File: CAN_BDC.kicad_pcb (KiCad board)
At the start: 2 copper layers, 24.5 x 34 mm, 31 parts, among them P1 CONN_01X02, P2 CONN_01X05, P4 CONN_01X04, P5 CONN_01X04, P6 CONN_01X02, P7 CONN_01X04, P8 CONN_01X04, P9 CONN_01X02, U1 PSD2CAN, U2 SN65HVD232D, U3 POLOLU_DRV8825/DRV8801, U4 STM32F042G4U6, U5 Mini-360, U6 MCP1700T-3302E/TT

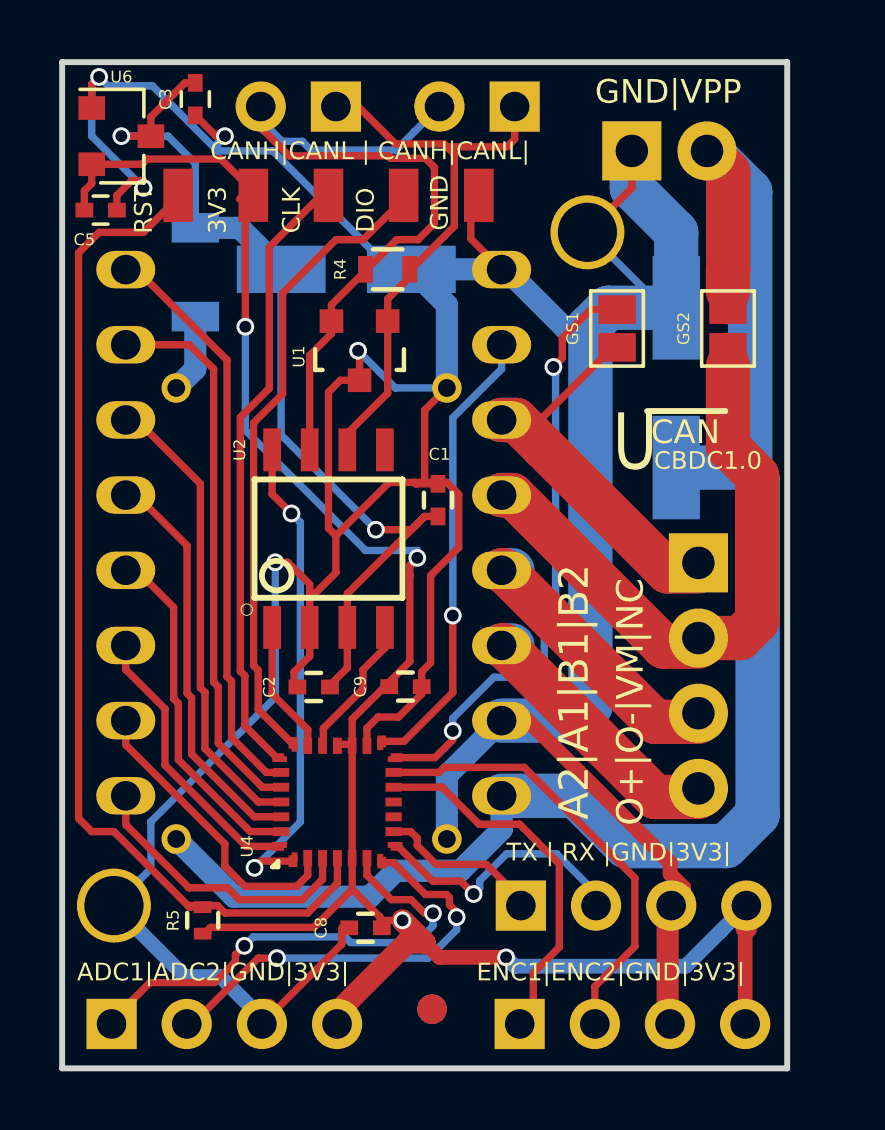
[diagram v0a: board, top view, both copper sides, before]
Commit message: Gerber Files generation
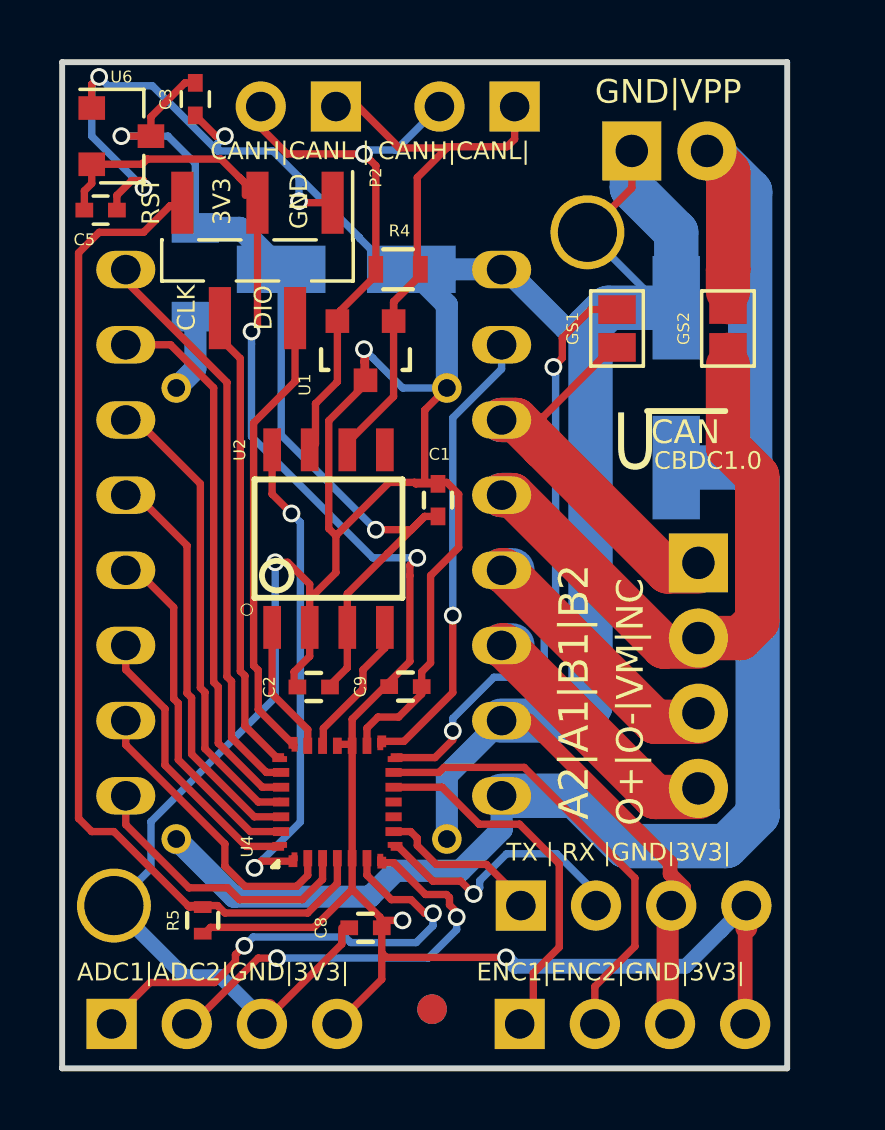
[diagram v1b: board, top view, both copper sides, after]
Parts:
- P2: footprint usb_ccb_custom:swd_smd_conn5 -> Pin_Headers:Pin_Header_Straight_1x05_Pitch1.27mm_SMD_Pin1Left
- moved P2 4.28 mm to (145.3, 85.0), turned to 270 degrees
- moved R4 0.35 mm to (150.1, 85.3)
- moved U1 0.20 mm to (148.9, 88.1)
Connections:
- P2 pad 3: SW_CLK -> +3V3
- P2 pad 4: +3V3 -> SW_CLK
- U2 pad 5: (no net) -> Net-(U2-Pad5)
- U4 pad 10: (no net) -> Net-(U4-Pad10)
- U4 pad 11: (no net) -> Net-(U4-Pad11)
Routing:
- net Net-(P1-Pad2): track 27.2 -> 19.4 mm, vias 0 -> 1
- net SW_DIO: track 21.7 -> 15.6 mm
- net SW_CLK: track 20.8 -> 15.7 mm
- net Net-(P1-Pad1): track 20.6 -> 22.1 mm
- net GND: track 153.2 -> 152.8 mm, vias 5 -> 6
